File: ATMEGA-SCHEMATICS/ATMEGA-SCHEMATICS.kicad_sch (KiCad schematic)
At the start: 0 parts

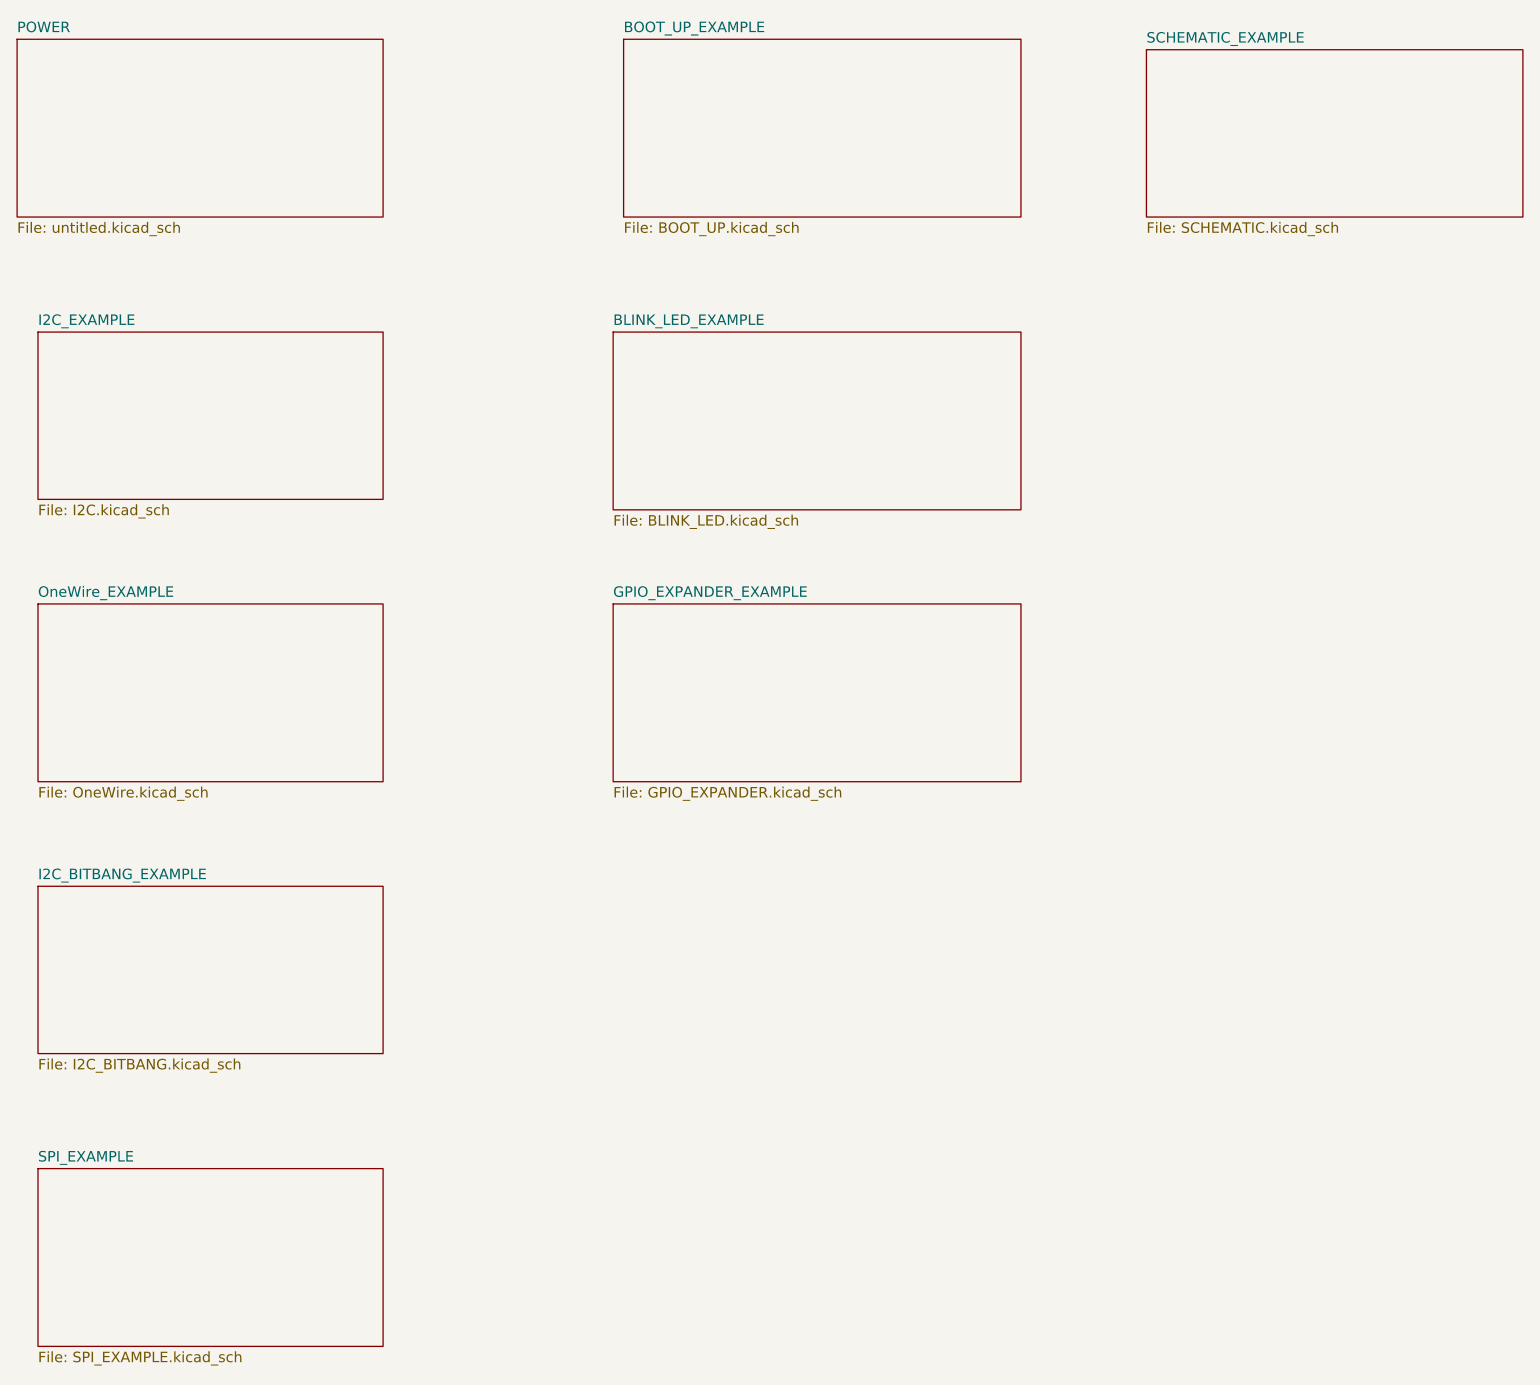
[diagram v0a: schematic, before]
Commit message: .
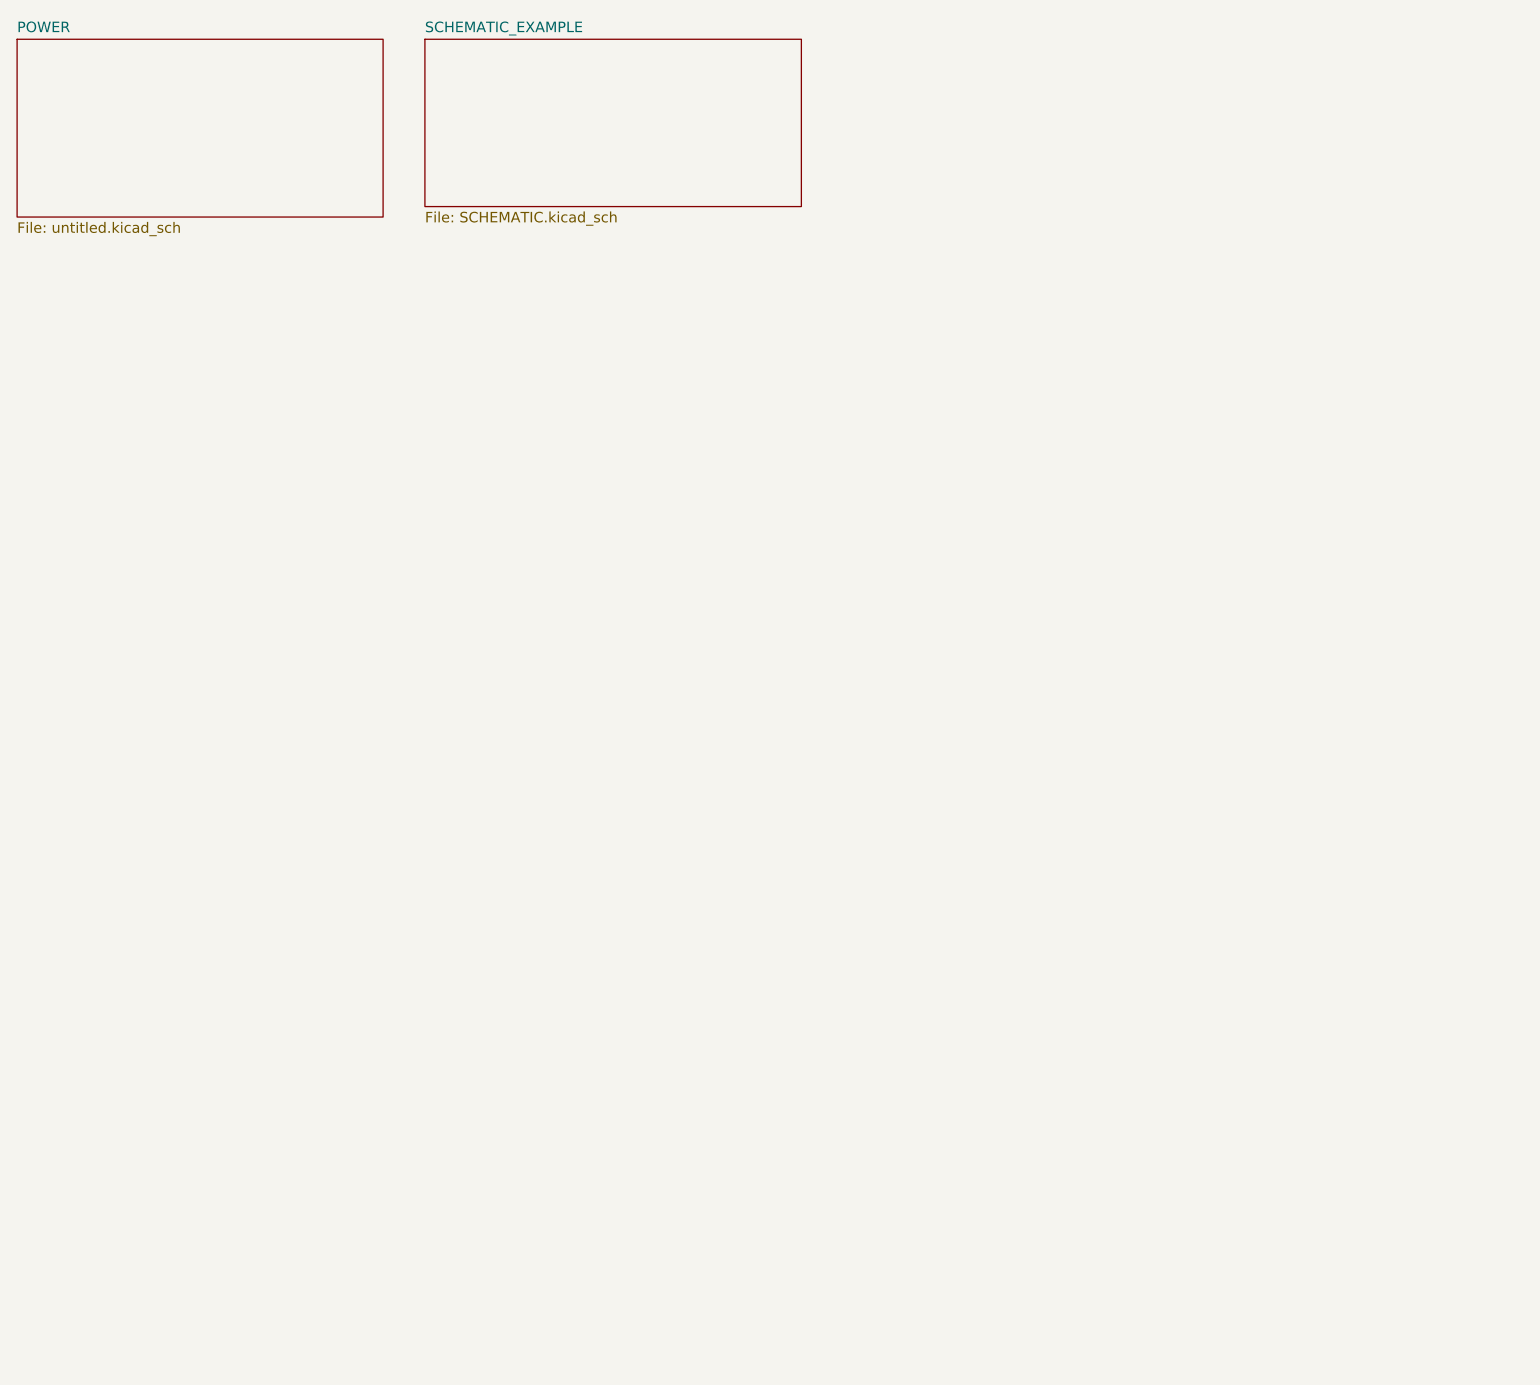
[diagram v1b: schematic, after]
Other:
- removed sheet BLINK_LED_EXAMPLE
- removed sheet BOOT_UP_EXAMPLE
- removed sheet GPIO_EXPANDER_EXAMPLE
- removed sheet I2C_BITBANG_EXAMPLE
- removed sheet I2C_EXAMPLE
- removed sheet OneWire_EXAMPLE
- removed sheet SPI_EXAMPLE
